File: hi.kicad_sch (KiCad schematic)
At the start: 4 parts, among them J1 Power, J2 Digital/PWM, J3 Analog, J4 Digital/PWM

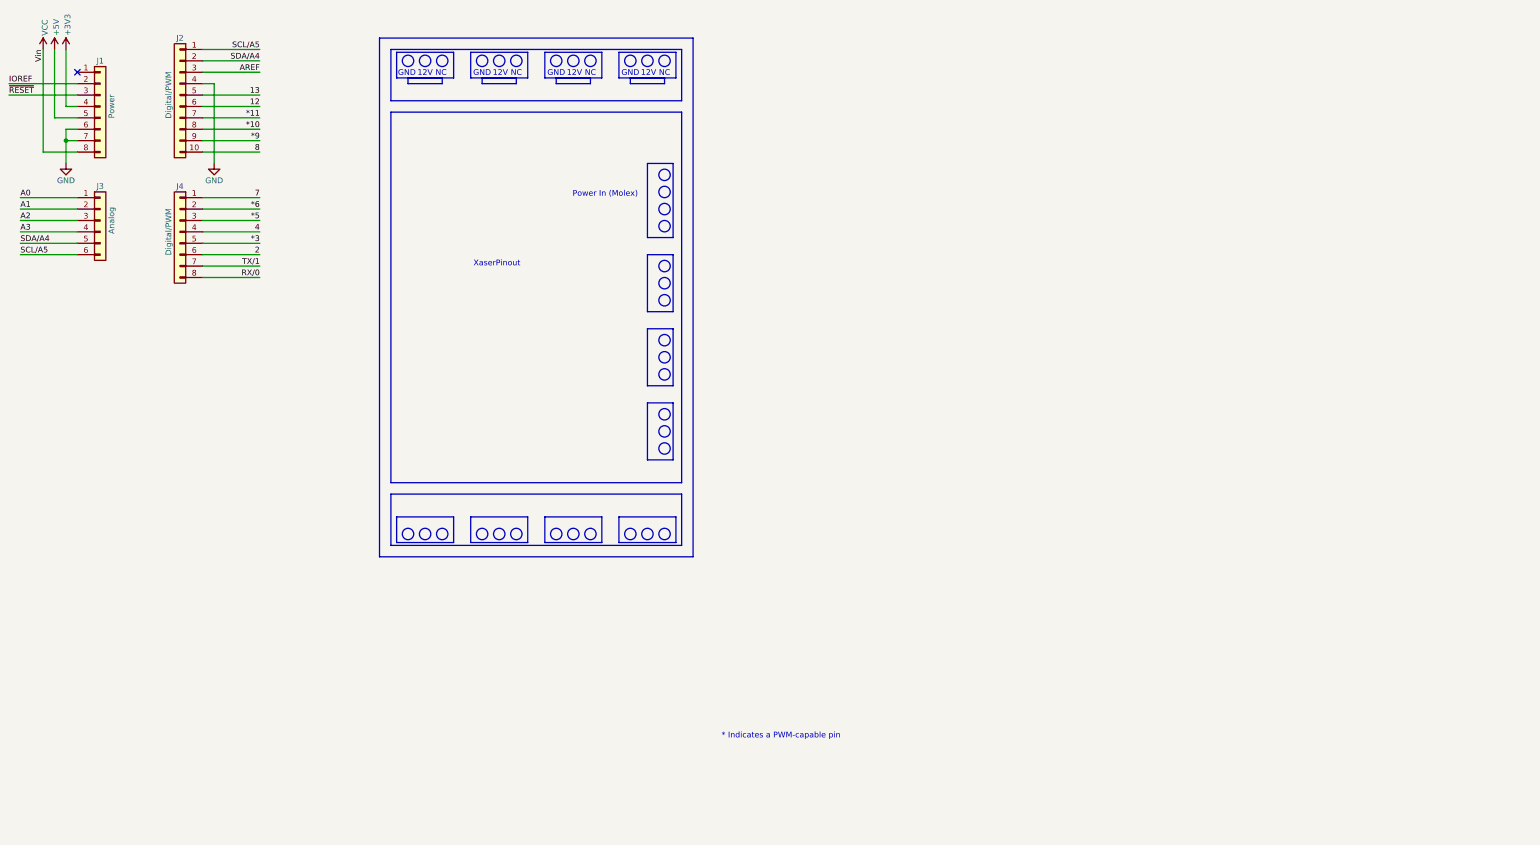
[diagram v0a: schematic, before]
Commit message: hi
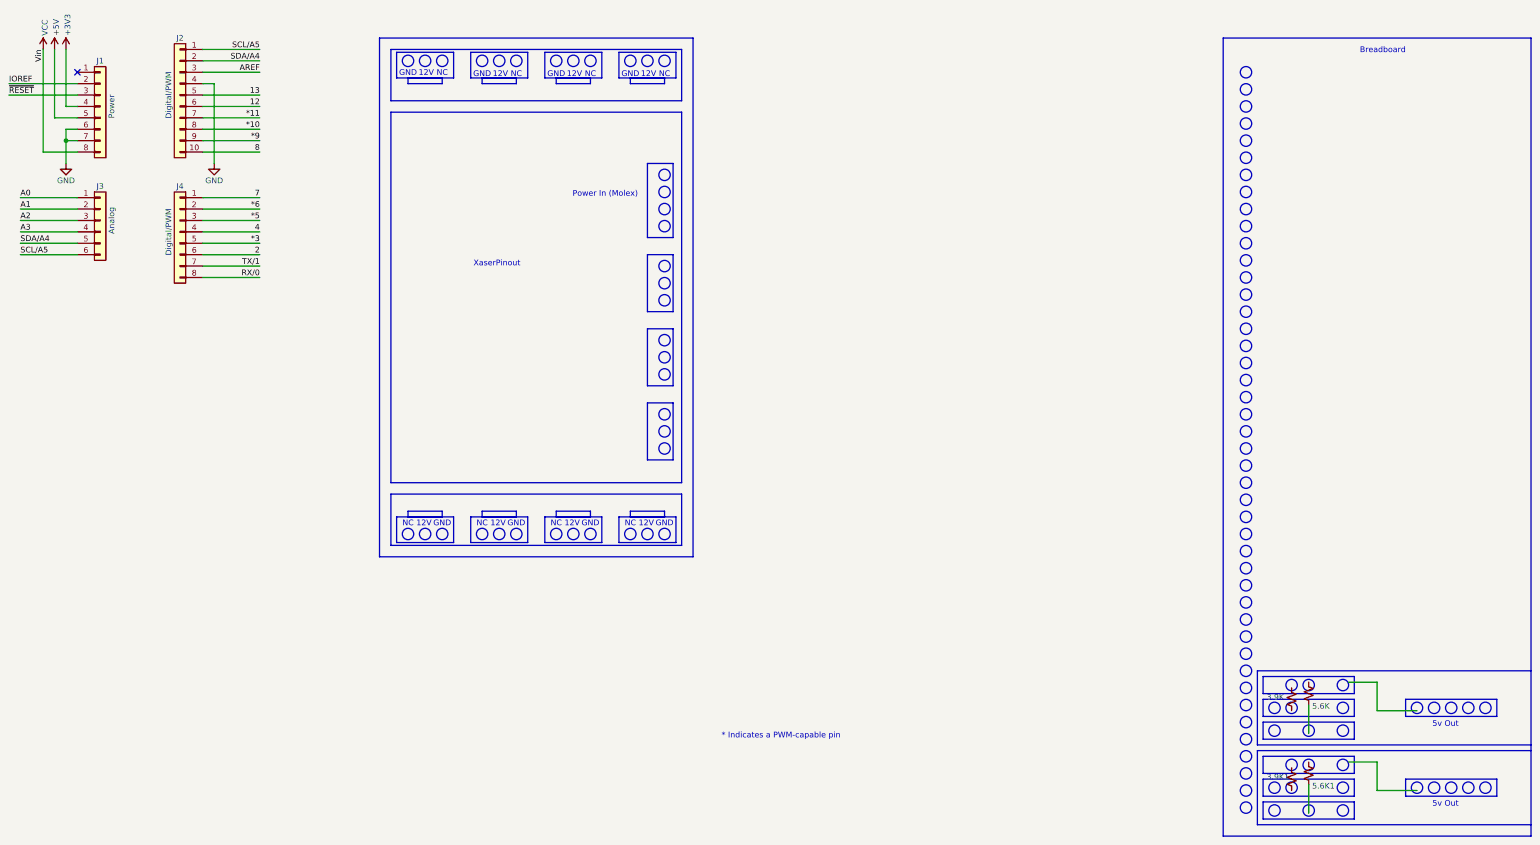
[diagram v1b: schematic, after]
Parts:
- added 3.9K, 3.9K1, 5.6K, 5.6K1: R_Small_US, symbol Device:R_Small_US
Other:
- note added: "5v Out"
- note added: "Breadboard"
